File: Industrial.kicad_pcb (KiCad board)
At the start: 2 copper layers, 101.6 x 39.4 mm, 17 parts, among them J1 ASC712, J2 INA219, J3 Corriente, Q1 TIC106, U1 H11AA1, U2 MOC3052M, U3 Esp32

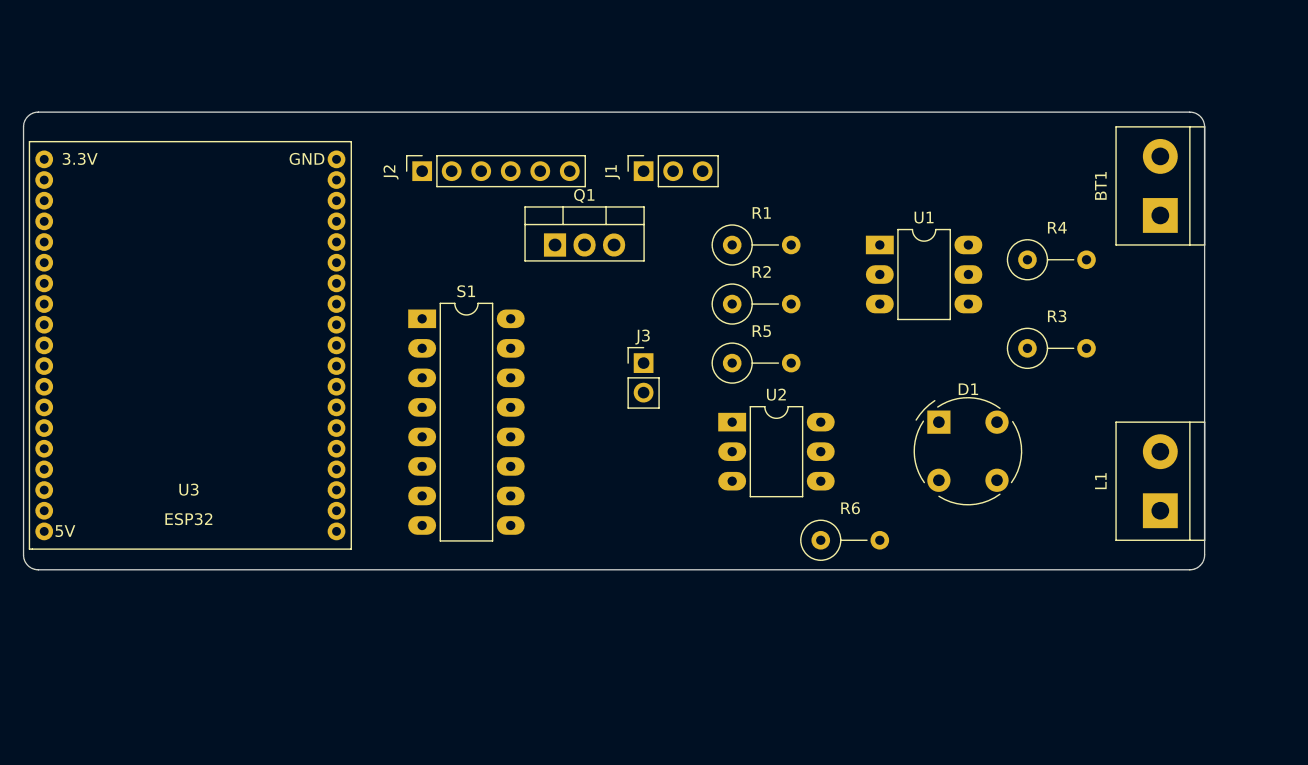
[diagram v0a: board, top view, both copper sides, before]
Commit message: fix pcb
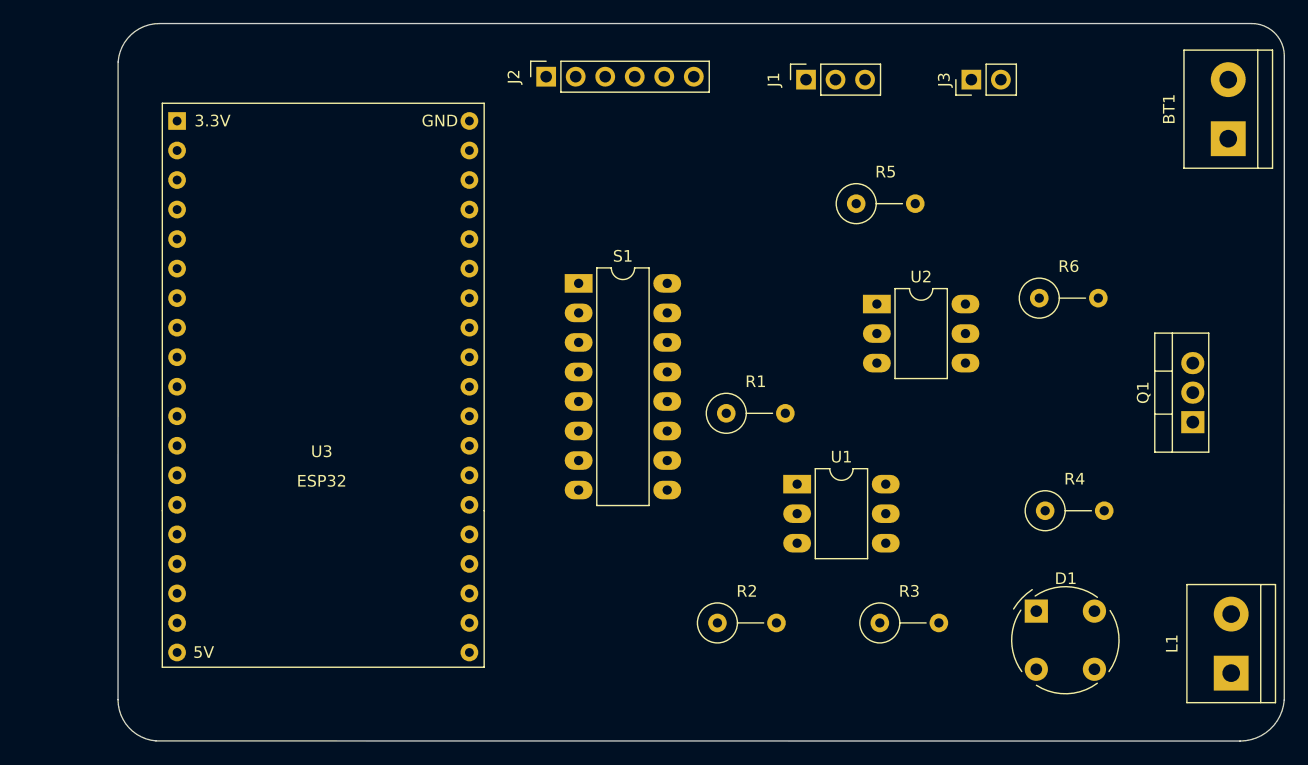
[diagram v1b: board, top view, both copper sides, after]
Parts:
- moved Q1 56.9 mm to (194.6, 111.8), turned to 90 degrees
- moved J3 37.3 mm to (175.5, 82.3), turned to 90 degrees
- moved R6 28.1 mm to (181.4, 101.1)
- moved R2 27.5 mm to (153.7, 129.0)
- moved R3 26.8 mm to (167.6, 129.0)
- moved U1 21.8 mm to (160.5, 117.1)
- moved R4 21.6 mm to (181.9, 119.4)
- moved D1 18.3 mm to (181.1, 128.0)
- moved R5 17.4 mm to (165.6, 93.0)
- moved U2 16.1 mm to (167.4, 101.6)
- moved J1 16.0 mm to (161.3, 82.3)
- moved L1 15.2 mm to (197.9, 133.3)
- moved R1 14.5 mm to (154.4, 111.0)
- moved S1 13.8 mm to (141.7, 99.8)
- moved J2 13.4 mm to (138.9, 82.0)
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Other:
- board size 101.6 x 39.4 mm -> 100.3 x 61.7 mm
